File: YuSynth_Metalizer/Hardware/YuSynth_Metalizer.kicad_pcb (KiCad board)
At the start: 2 copper layers, 29 x 108 mm, 79 parts, among them J37 CV1, J38 CV2, J39 In, J40 Out, Q1 BC547, Q10 BC547, Q11 BC557, Q12 BC547, Q2 BC547, Q3 BC547, Q4 BC547, Q5 BC557, Q6 BC547, Q7 BC557, Q8 BC547, Q9 BC557, U1 TL072, U2 TL074

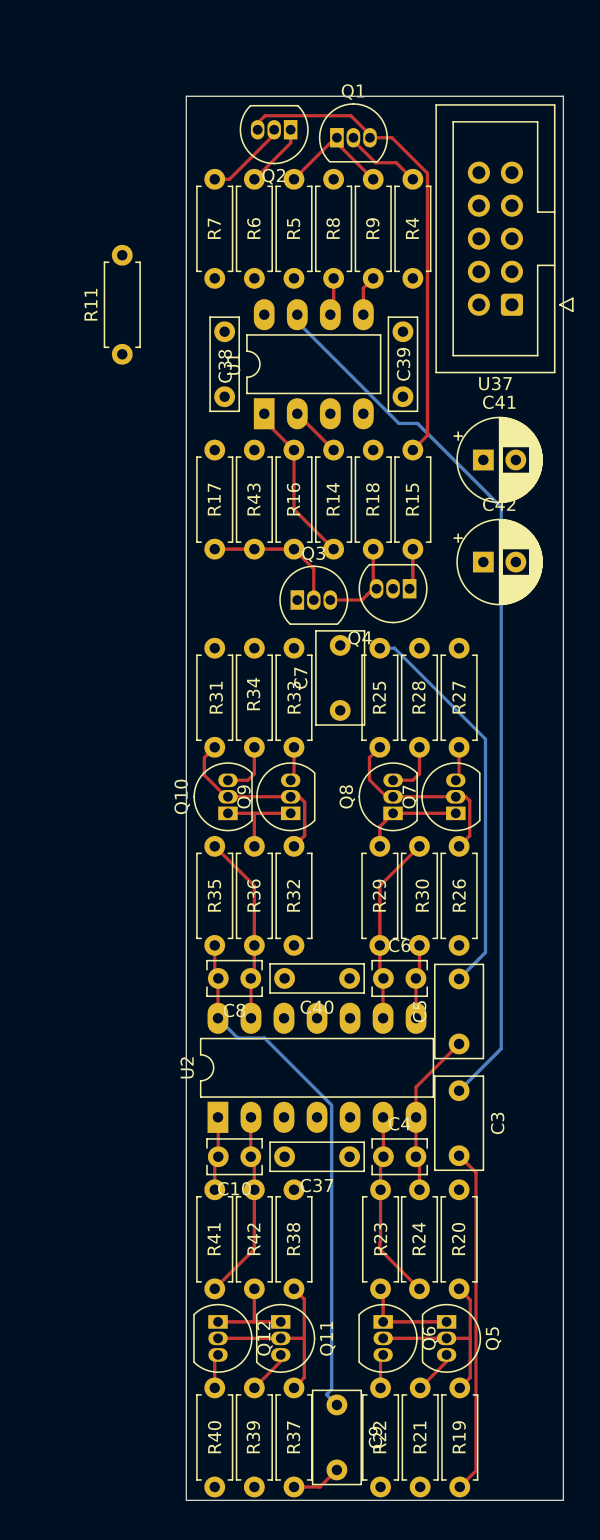
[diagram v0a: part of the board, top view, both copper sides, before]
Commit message: Main board & panel nearly done
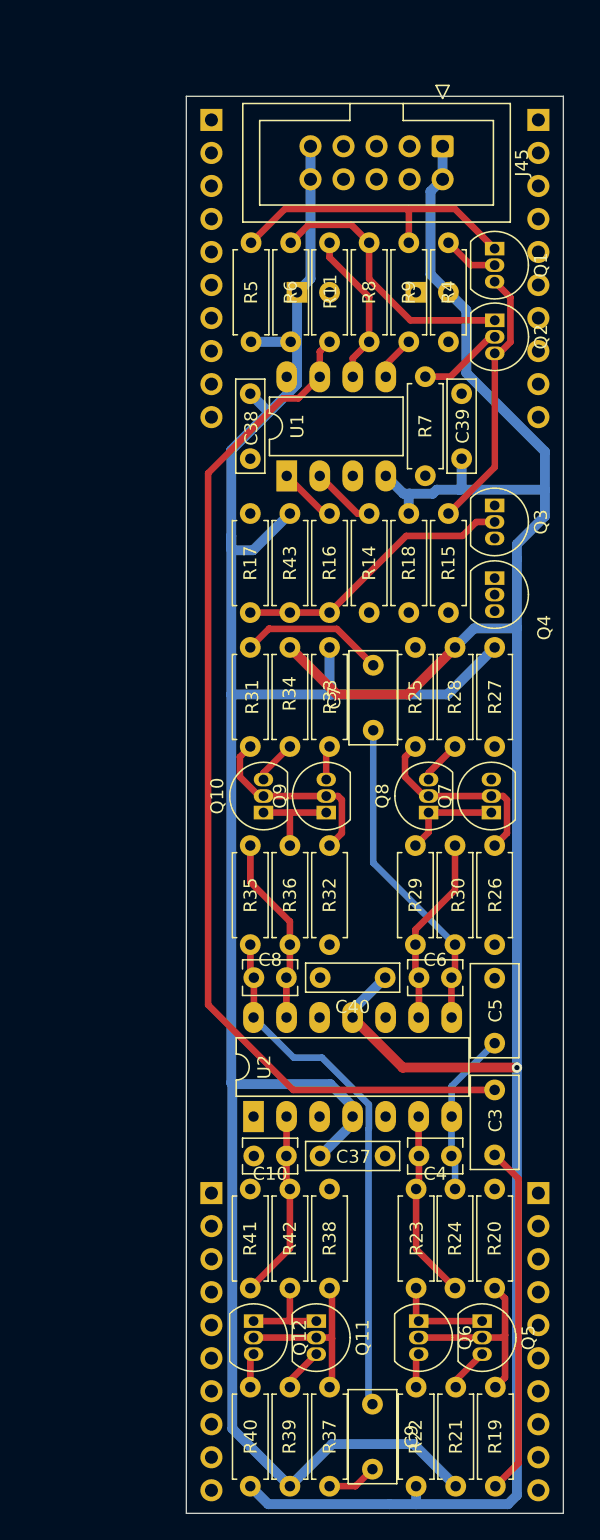
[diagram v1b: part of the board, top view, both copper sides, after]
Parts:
- removed U37: ~, Connector_IDC:IDC-Header_2x05_P2.54mm_Vertical
- added J41: Conn_01x10, Connector_PinHeader_2.54mm:PinHeader_1x10_P2.54mm_Vertical, B.Cu at (201.9, 51.8)
- added J42: Conn_01x10, Connector_PinHeader_2.54mm:PinHeader_1x10_P2.54mm_Vertical, B.Cu at (201.9, 134.4)
- added J43: Conn_01x10, Connector_PinHeader_2.54mm:PinHeader_1x10_P2.54mm_Vertical, B.Cu at (227.1, 134.4)
- added J44: Conn_01x10, Connector_PinHeader_2.54mm:PinHeader_1x10_P2.54mm_Vertical, B.Cu at (227.1, 51.8)
- added J45: Conn_02x05_Odd_Even, Connector_IDC:IDC-Header_2x05_P2.54mm_Vertical, F.Cu at (219.7, 53.8)
- C41, C42: moved to B.Cu
- moved R7 22.2 mm to (218.4, 71.6)
- moved Q2 21.5 mm to (223.7, 67.2), turned to -90 degrees
- moved C42 21.4 mm to (217.7, 65.1)
- moved C41 19.3 mm to (208.5, 65.1)
- moved R11 18.1 mm to (211.0, 61.3), turned to -90 degrees
- moved Q3 16.8 mm to (223.7, 81.5), turned to -90 degrees
- moved Q1 14.8 mm to (223.7, 61.7), turned to -90 degrees
- moved Q4 6.60 mm to (223.7, 87.1), turned to -90 degrees
- moved C39 6.56 mm to (221.2, 77.9)
- moved R5 5.89 mm to (205.0, 68.9)
- moved R6 5.62 mm to (208.0, 68.9)
- moved R14 5.59 mm to (214.1, 82.1)
- moved R16 5.59 mm to (211.0, 82.1)
- moved R17 5.59 mm to (204.9, 89.7)
- moved R18 5.59 mm to (217.1, 89.7)
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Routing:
- net -12V: track 0.00 -> 187.8 mm, vias 0 -> 1
- net +12V: track 0.00 -> 176.3 mm
- net Net-(C5-Pad2): track 30.3 -> 0.00 mm
- net Net-(C6-Pad2): track 5.72 -> 24.8 mm
- net Net-(Q1-E): track 37.5 -> 20.5 mm
- net Net-(Q2-C): track 4.97 -> 20.9 mm
- net Net-(Q1-C): track 8.98 -> 23.7 mm
- net Net-(C3-Pad1): track 68.4 -> 80.3 mm
- net Net-(C7-Pad2): track 0.00 -> 11.2 mm
- net Net-(Q3-B): track 10.6 -> 21.7 mm
- net Net-(U1B--): track 2.90 -> 12.1 mm
- net Net-(R14-Pad2): track 12.6 -> 4.49 mm
- net Net-(Q3-E): track 6.71 -> 0.00 mm
- net Net-(C10-Pad2): track 5.70 -> 0.00 mm
- net Net-(Q4-C): track 3.26 -> 0.00 mm
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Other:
- board size 29 x 108 mm -> 29 x 109 mm
